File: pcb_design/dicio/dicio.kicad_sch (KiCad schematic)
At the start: 76 parts, among them J1 Conn_02x03_Counter_Clockwise, J2 Conn_01x06_Female, J3 USB_C_Receptacle, J4 Micro_SD_Card, J5 USB_C_Receptacle, J6 USB_C_Receptacle, J7 Conn_02x13_Odd_Even, J8 USB_C_Receptacle, Q1 Q_NMOS_GSD, SW1 SW_SPST, SW2 SW_SPST, U1 dsPIC33EP256MU806, U2 MCP2542FD, U3 S70FL01GS, U4 TPS737, U5 SiP32431, U6 SiP32431, U7 ADM7170, Y1 Crystal_GND24, Y2 Crystal_GND24

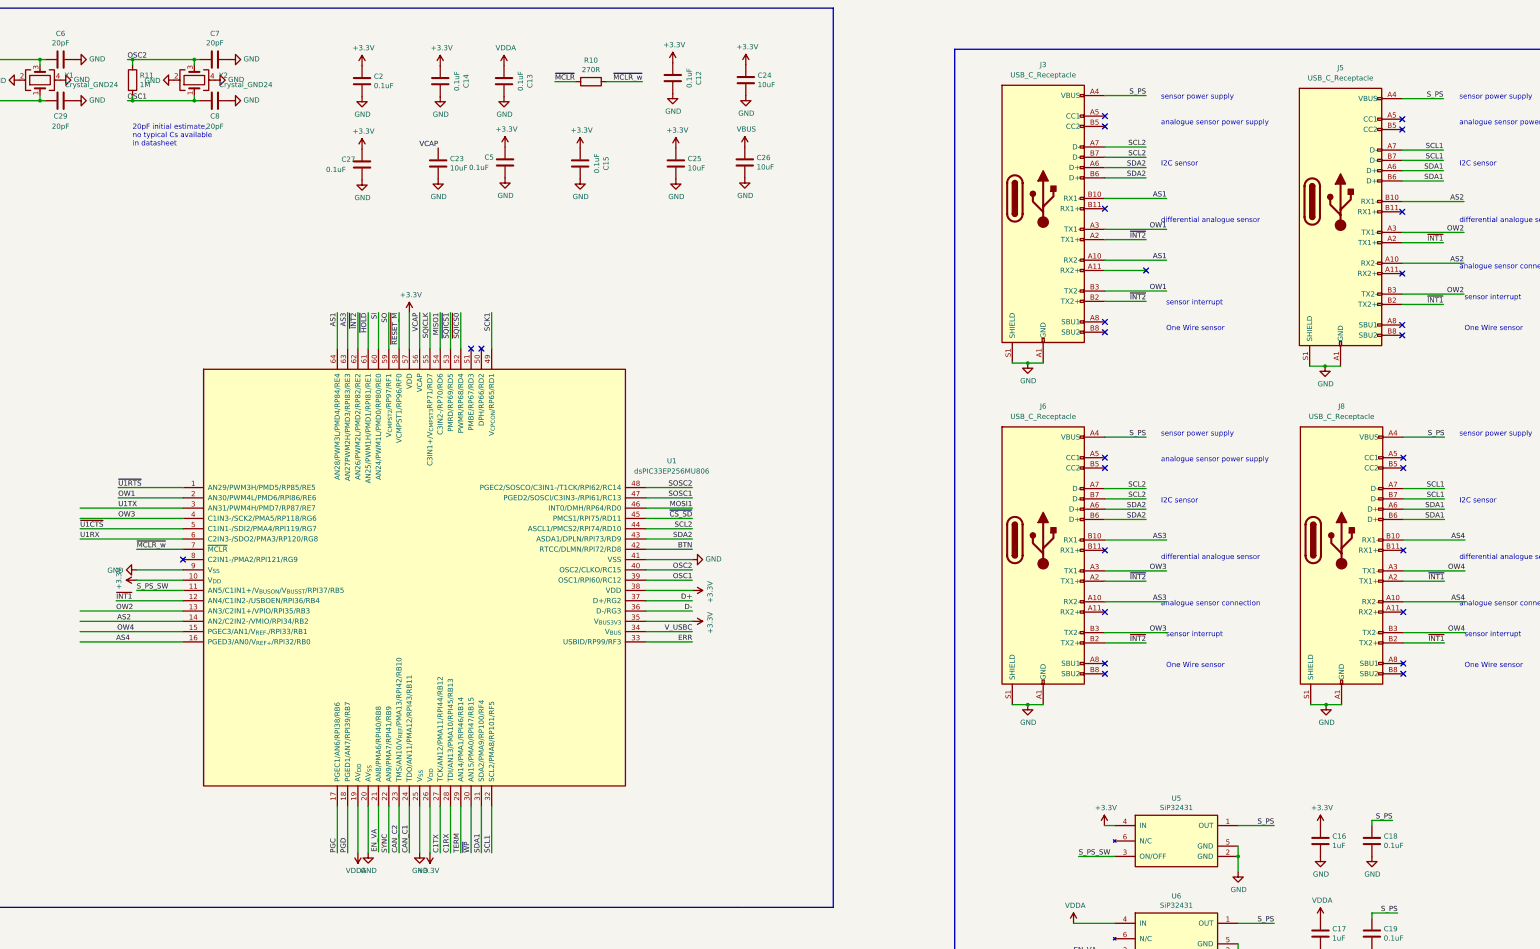
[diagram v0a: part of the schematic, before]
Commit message: Improved design.
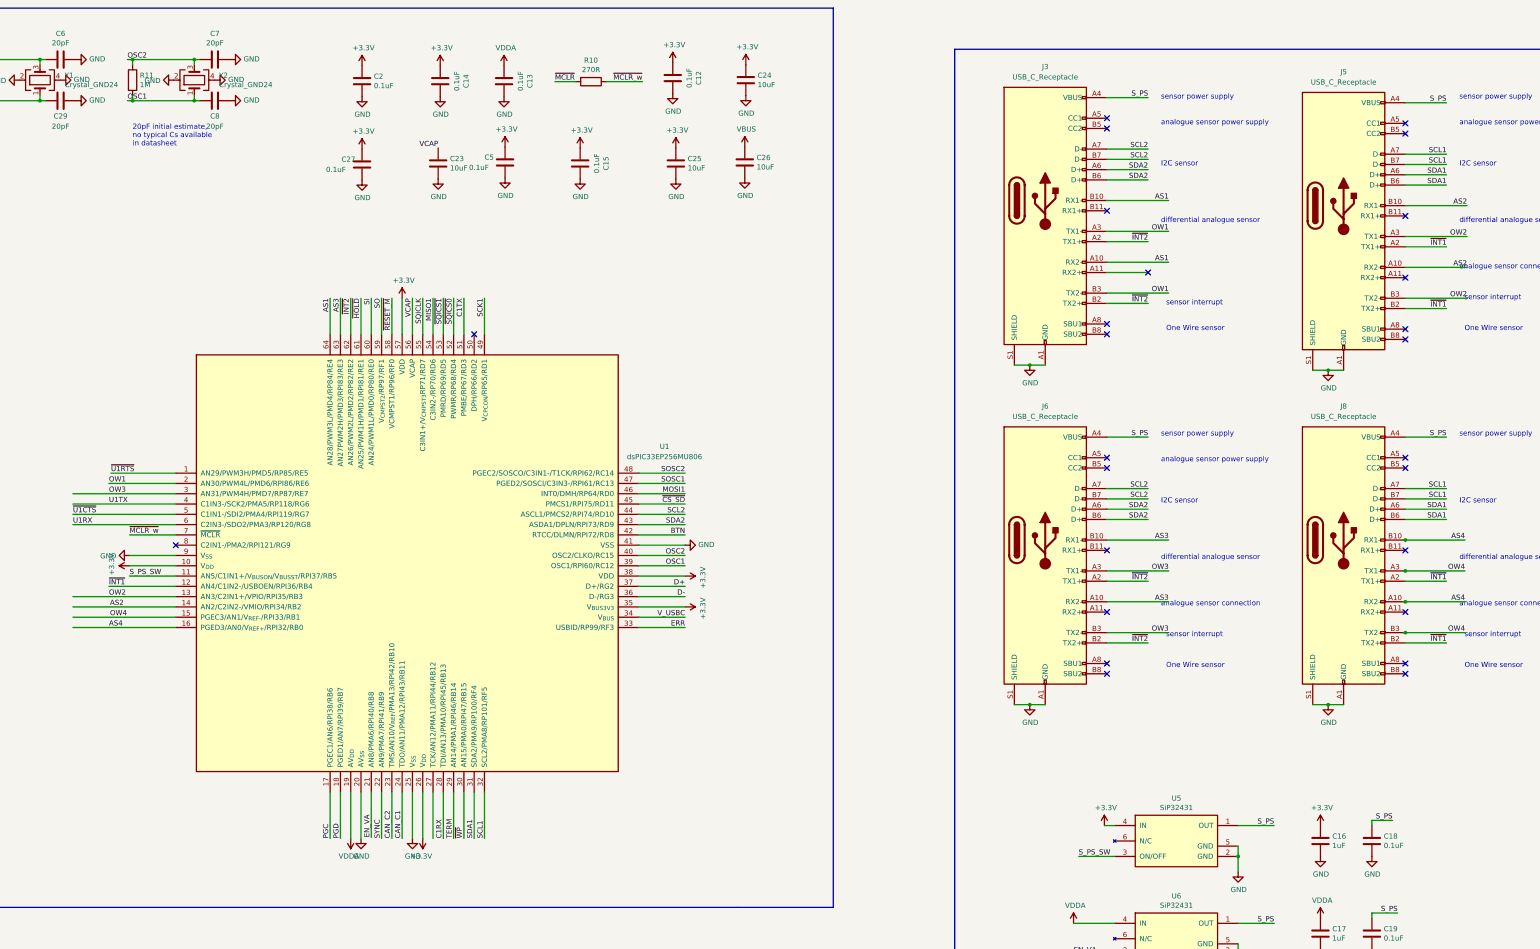
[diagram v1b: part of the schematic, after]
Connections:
- net C1TX: now also U1.51 (PMBE/RP67/RD3); no longer U1.27 (TCK/AN12/PMA11/RPI44/RB12)
- net OW3: now also U1.3 (AN31/PWM4H/PMD7/RP87/RE7); no longer U1.4 (C1IN3-/SCK2/PMA5/RP118/RG6)
- net U1TX: now also U1.4 (C1IN3-/SCK2/PMA5/RP118/RG6); no longer U1.3 (AN31/PWM4H/PMD7/RP87/RE7)
- no-connect marks 39 -> 38
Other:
- moved on the sheet: J3, J5, J6, J8, U1
